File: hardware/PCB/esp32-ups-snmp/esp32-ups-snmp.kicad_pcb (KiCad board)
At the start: 2 copper layers, 23.7 x 90.3 mm, 2 parts, among them J1 USB_A

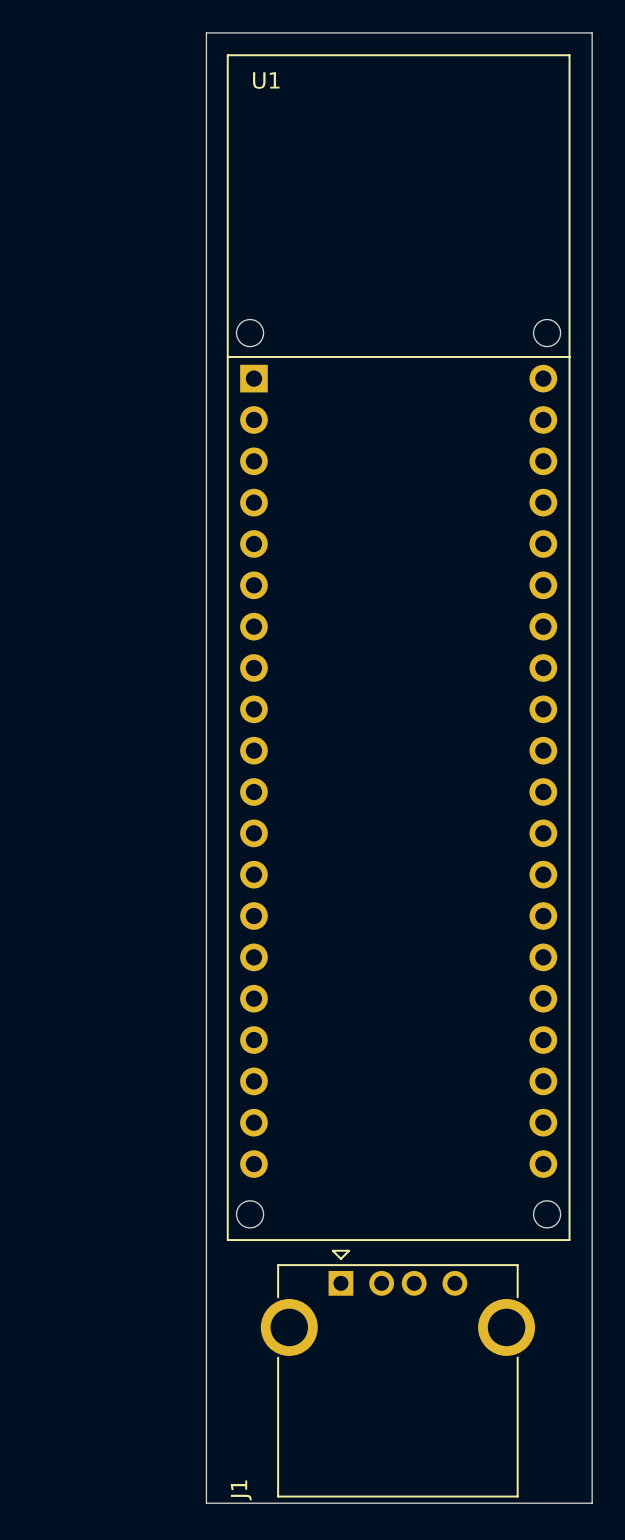
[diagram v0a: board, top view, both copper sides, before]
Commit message: WIP on HTTP OTA
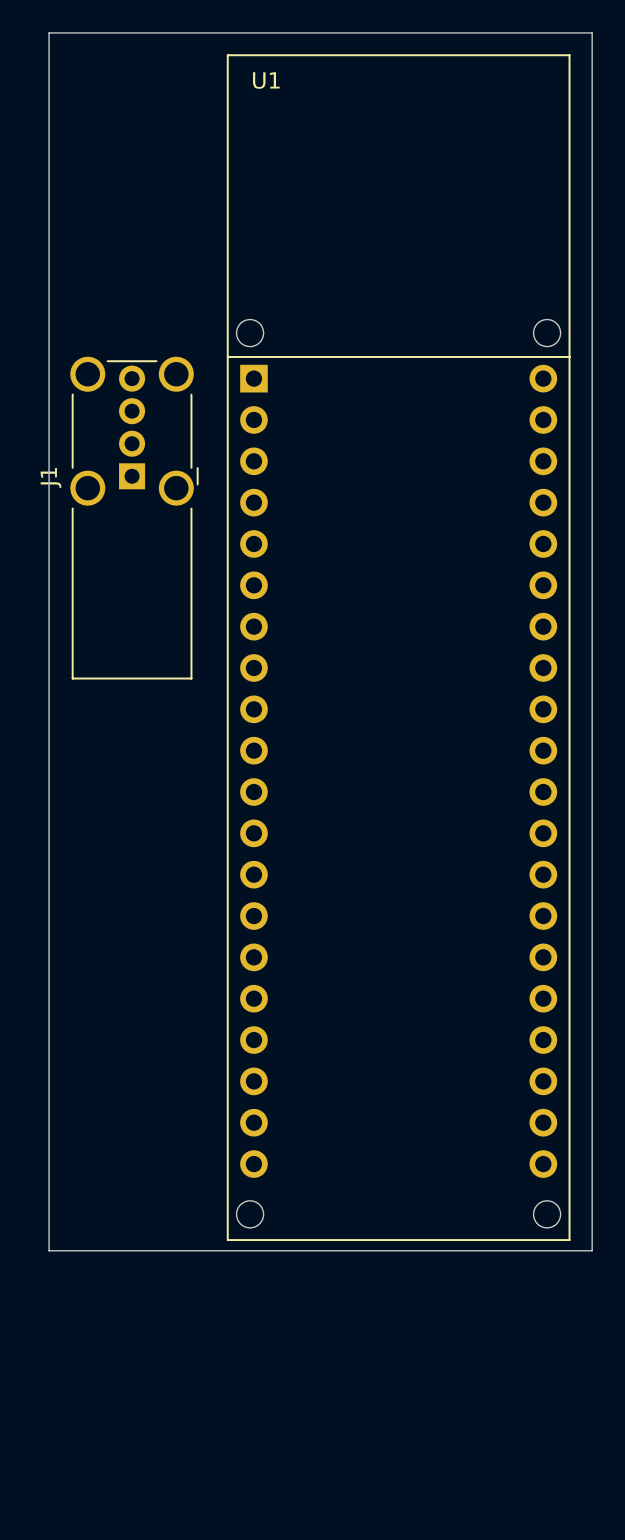
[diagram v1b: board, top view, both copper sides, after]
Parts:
- J1: footprint Connector_USB:USB_A_Kycon_KUSBX-AS1N-B_Horizontal -> Connector_USB:USB_A_Wuerth_614004134726_Horizontal
- moved J1 51.2 mm to (121.8, 83.7), turned to 90 degrees
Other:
- board size 23.7 x 90.3 mm -> 33.4 x 74.8 mm
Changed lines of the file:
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@@
 		)
 	)
-	(footprint "Connector_USB:USB_A_Kycon_KUSBX-AS1N-B_Horizontal"
+	(footprint "Connector_USB:USB_A_Wuerth_614004134726_Horizontal"
 		(layer "F.Cu")
-		(at 134.585 133.29)
-		(descr "Kycon, USB-A receptacle, through-hole, https://www.kycon.com/Catalog_PDF/KUSBX.pdf'")
-		(tags "USB-A receptacle horizontal THT")
+		(at 121.75 83.7 90)
+		(descr "USB A connector https://www.we-online.com/catalog/datasheet/614004134726.pdf")
+		(tags "USB_A Female Connector receptacle")
 		(property "Reference" "J1"
-			(at -6.225 12.62 90)
+			(at 0 -5.08 90)
 			(layer "F.SilkS")
 			(effects
@@
 		)
 		(property "Value" "USB_A"
-			(at 0 7 0)
+			(at 0 5.08 90)
 			(layer "F.Fab")
 			(effects
@@
 			)
 		)
-		(property "Footprint" "Connector_USB:USB_A_Kycon_KUSBX-AS1N-B_Horizontal"
-			(at 3.5 0 0)
+		(property "Footprint" "Connector_USB:USB_A_Wuerth_614004134726_Horizontal"
+			(at 0 0 90)
+			(unlocked yes)
 			(layer "F.Fab")
 			(hide yes)
@@
 		)
 		(property "Datasheet" ""
-			(at 0 15 0)
+			(at 0 0 90)
+			(unlocked yes)
 			(layer "F.Fab")
 			(hide yes)
@@
 		)
 		(property "Description" "USB Type A connector"
-			(at 0 9 0)
+			(at 0 0 90)
+			(unlocked yes)
 			(layer "F.Fab")
 			(hide yes)
@@
 		(attr through_hole)
 		(fp_line
-			(start -3.86 -1.12)
-			(end -3.86 0.86)
-			(stroke
-				(width 0.12)
-				(type solid)
-			)
-			(layer "F.SilkS")
-		)
-		(fp_line
-			(start -3.86 -1.12)
-			(end 10.86 -1.12)
-			(stroke
-				(width 0.12)
-				(type solid)
-			)
-			(layer "F.SilkS")
-		)
-		(fp_line
-			(start -3.86 4.56)
-			(end -3.86 13.1)
-			(stroke
-				(width 0.12)
-				(type solid)
-			)
-			(layer "F.SilkS")
-		)
-		(fp_line
-			(start -3.86 13.1)
-			(end 10.86 13.1)
-			(stroke
-				(width 0.12)
-				(type solid)
-			)
-			(layer "F.SilkS")
-		)
-		(fp_line
-			(start -0.5 -2)
-			(end 0 -1.5)
-			(stroke
-				(width 0.12)
-				(type solid)
-			)
-			(layer "F.SilkS")
-		)
-		(fp_line
-			(start 0 -1.5)
-			(end 0.5 -2)
-			(stroke
-				(width 0.12)
-				(type solid)
-			)
-			(layer "F.SilkS")
-		)
-		(fp_line
-			(start 0.5 -2)
-			(end -0.5 -2)
-			(stroke
-				(width 0.12)
-				(type solid)
-			)
-			(layer "F.SilkS")
-		)
-		(fp_line
-			(start 10.86 0.86)
-			(end 10.86 -1.12)
-			(stroke
-				(width 0.12)
-				(type solid)
-			)
-			(layer "F.SilkS")
-		)
-		(fp_line
-			(start 10.86 4.56)
-			(end 10.86 13.1)
-			(stroke
-				(width 0.12)
-				(type solid)
-			)
-			(layer "F.SilkS")
-		)
-		(fp_line
-			(start -5.43 -1.51)
-			(end -5.43 13.49)
+			(start 0.52 -3.65)
+			(end 5.02 -3.65)
+			(stroke
+				(width 0.12)
+				(type solid)
+			)
+			(layer "F.SilkS")
+		)
+		(fp_line
+			(start -12.43 -3.65)
+			(end -1.98 -3.65)
+			(stroke
+				(width 0.12)
+				(type solid)
+			)
+			(layer "F.SilkS")
+		)
+		(fp_line
+			(start -12.43 -3.65)
+			(end -12.43 3.65)
+			(stroke
+				(width 0.12)
+				(type solid)
+			)
+			(layer "F.SilkS")
+		)
+		(fp_line
+			(start 7.07 -1.5)
+			(end 7.07 1.5)
+			(stroke
+				(width 0.12)
+				(type solid)
+			)
+			(layer "F.SilkS")
+		)
+		(fp_line
+			(start 0.52 3.65)
+			(end 5.02 3.65)
+			(stroke
+				(width 0.12)
+				(type solid)
+			)
+			(layer "F.SilkS")
+		)
+		(fp_line
+			(start -12.43 3.65)
+			(end -1.98 3.65)
+			(stroke
+				(width 0.12)
+				(type solid)
+			)
+			(layer "F.SilkS")
+		)
+		(fp_line
+			(start -0.5 4.03)
+			(end 0.5 4.03)
+			(stroke
+				(width 0.12)
+				(type solid)
+			)
+			(layer "F.SilkS")
+		)
+		(fp_line
+			(start 7.85 -4.3)
+			(end 7.85 4.3)
 			(stroke
 				(width 0.05)
@@
 		)
 		(fp_line
-			(start -5.43 -1.51)
-			(end 12.43 -1.51)
+			(start -12.83 -4.3)
+			(end 7.85 -4.3)
 			(stroke
 				(width 0.05)
@@
 		)
 		(fp_line
-			(start 12.43 -1.51)
-			(end 12.43 13.49)
+			(start 7.85 4.3)
+			(end -12.83 4.3)
 			(stroke
 				(width 0.05)
@@
 		)
 		(fp_line
-			(start 12.43 13.49)
-			(end -5.43 13.49)
+			(start -12.83 4.3)
+			(end -12.83 -4.3)
 			(stroke
 				(width 0.05)
@@
 		)
 		(fp_line
-			(start -3.75 -0.13)
-			(end -3.75 12.99)
-			(stroke
-				(width 0.1)
-				(type solid)
-			)
-			(layer "F.Fab")
-		)
-		(fp_line
-			(start -3.75 12.99)
-			(end 10.75 12.99)
-			(stroke
-				(width 0.1)
-				(type solid)
-			)
-			(layer "F.Fab")
-		)
-		(fp_line
-			(start -2.87 -1.01)
-			(end -3.75 -0.13)
-			(stroke
-				(width 0.1)
-				(type solid)
-			)
-			(layer "F.Fab")
-		)
-		(fp_line
-			(start -2.87 -1.01)
-			(end 10.75 -1.01)
-			(stroke
-				(width 0.1)
-				(type solid)
-			)
-			(layer "F.Fab")
-		)
-		(fp_line
-			(start 10.75 -1.01)
-			(end 10.75 12.99)
+			(start 6.97 -3.55)
+			(end 6.97 3.55)
+			(stroke
+				(width 0.1)
+				(type solid)
+			)
+			(layer "F.Fab")
+		)
+		(fp_line
+			(start -12.33 -3.55)
+			(end 6.97 -3.55)
+			(stroke
+				(width 0.1)
+				(type solid)
+			)
+			(layer "F.Fab")
+		)
+		(fp_line
+			(start 0 1.25)
+			(end 0.5 3.55)
+			(stroke
+				(width 0.1)
+				(type solid)
+			)
+			(layer "F.Fab")
+		)
+		(fp_line
+			(start 6.97 3.55)
+			(end -12.33 3.55)
+			(stroke
+				(width 0.1)
+				(type solid)
+			)
+			(layer "F.Fab")
+		)
+		(fp_line
+			(start -0.5 3.55)
+			(end 0 1.25)
+			(stroke
+				(width 0.1)
+				(type solid)
+			)
+			(layer "F.Fab")
+		)
+		(fp_line
+			(start -12.33 3.55)
+			(end -12.33 -3.55)
 			(stroke
 				(width 0.1)
@@
 		)
 		(fp_text user "${REFERENCE}"
-			(at 3 5 0)
+			(at -2.855 0 90)
 			(layer "F.Fab")
 			(effects
@@
 		)
 		(pad "1" thru_hole rect
-			(at 0 0)
-			(size 1.524 1.524)
+			(at 0 0 90)
+			(size 1.6 1.6)
 			(drill 0.92)
 			(layers "*.Cu" "*.Mask")
@@
 		)
 		(pad "2" thru_hole circle
-			(at 2.5 0)
-			(size 1.524 1.524)
+			(at 2 0 90)
+			(size 1.6 1.6)
 			(drill 0.92)
 			(layers "*.Cu" "*.Mask")
@@
 		)
 		(pad "3" thru_hole circle
-			(at 4.5 0)
-			(size 1.524 1.524)
+			(at 4 0 90)
+			(size 1.6 1.6)
 			(drill 0.92)
 			(layers "*.Cu" "*.Mask")
@@
 		)
 		(pad "4" thru_hole circle
-			(at 7 0)
-			(size 1.524 1.524)
+			(at 6 0 90)
+			(size 1.6 1.6)
 			(drill 0.92)
 			(layers "*.Cu" "*.Mask")
@@
 		)
 		(pad "5" thru_hole circle
-			(at -3.175 2.71)
-			(size 3.5 3.5)
-			(drill 2.3)
+			(at -0.73 -2.72 90)
+			(size 2.15 2.15)
+			(drill 1.5)
 			(layers "*.Cu" "*.Mask")
 			(remove_unused_layers no)
@@
 		)
 		(pad "5" thru_hole circle
-			(at 10.175 2.71)
-			(size 3.5 3.5)
-			(drill 2.3)
+			(at -0.73 2.72 90)
+			(size 2.15 2.15)
+			(drill 1.5)
 			(layers "*.Cu" "*.Mask")
 			(remove_unused_layers no)
@@
 			(pintype "passive")
 		)
-		(model "${KICAD8_3DMODEL_DIR}/Connector_USB.3dshapes/USB_A_Molex_67643_Horizontal.wrl"
+		(pad "5" thru_hole circle
+			(at 6.27 -2.72 90)
+			(size 2.15 2.15)
+			(drill 1.5)
+			(layers "*.Cu" "*.Mask")
+			(remove_unused_layers no)
+			(net 1 "GND")
+			(pinfunction "Shield")
+			(pintype "passive")
+		)
+		(pad "5" thru_hole circle
+			(at 6.27 2.72 90)
+			(size 2.15 2.15)
+			(drill 1.5)
+			(layers "*.Cu" "*.Mask")
+			(remove_unused_layers no)
+			(net 1 "GND")
+			(pinfunction "Shield")
+			(pintype "passive")
+		)
+		(model "${KIPRJMOD}/3D/Wurth_614004134726 (rev1).stp"
 			(offset
-				(xyz 0 0 0)
+				(xyz -2.5 0 7.5)
 			)
 			(scale
@@
 			)
 			(rotate
-				(xyz 0 0 0)
+				(xyz 180 0 0)
 			)
 		)
 	)
 	(gr_rect
-		(start 126.32 56.46)
-		(end 150.02 146.8)
+		(start 116.65 56.46)
+		(end 150.02 131.29)
 		(stroke
 			(width 0.05)
